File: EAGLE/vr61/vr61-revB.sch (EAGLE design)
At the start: 235 parts, among them J2 SM04B-SRSS-TB(LF)(SN), J6 MICROMOD-2222-C, Y1 74AHCT1G125

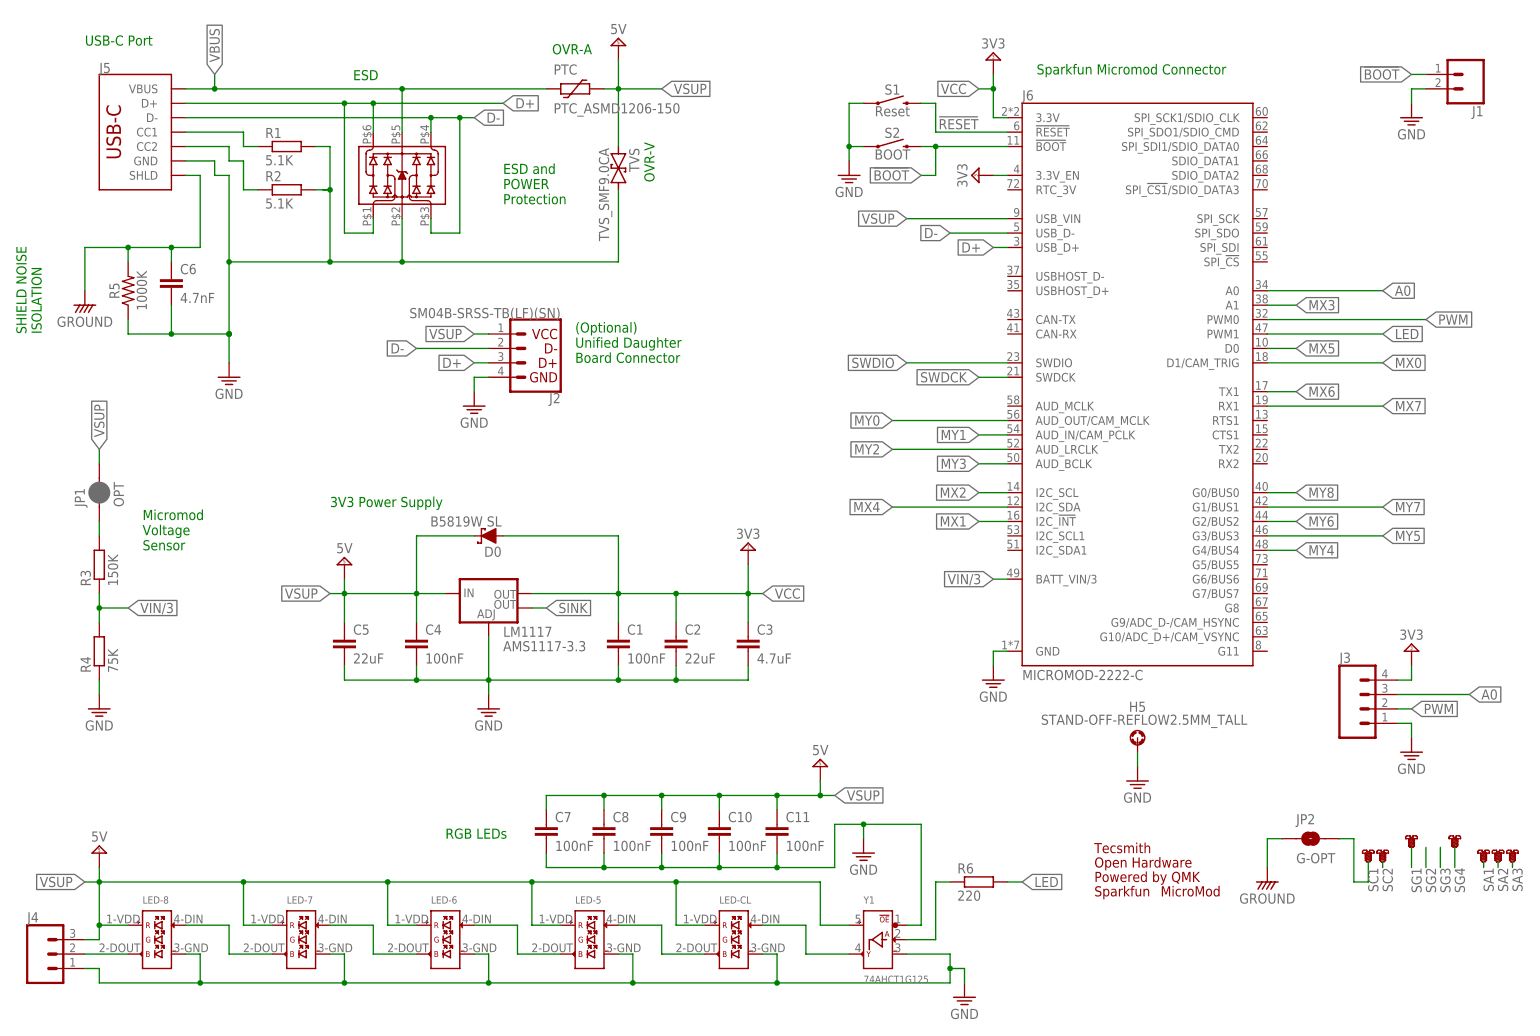
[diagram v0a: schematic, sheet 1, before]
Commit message: wip 2022-07-21
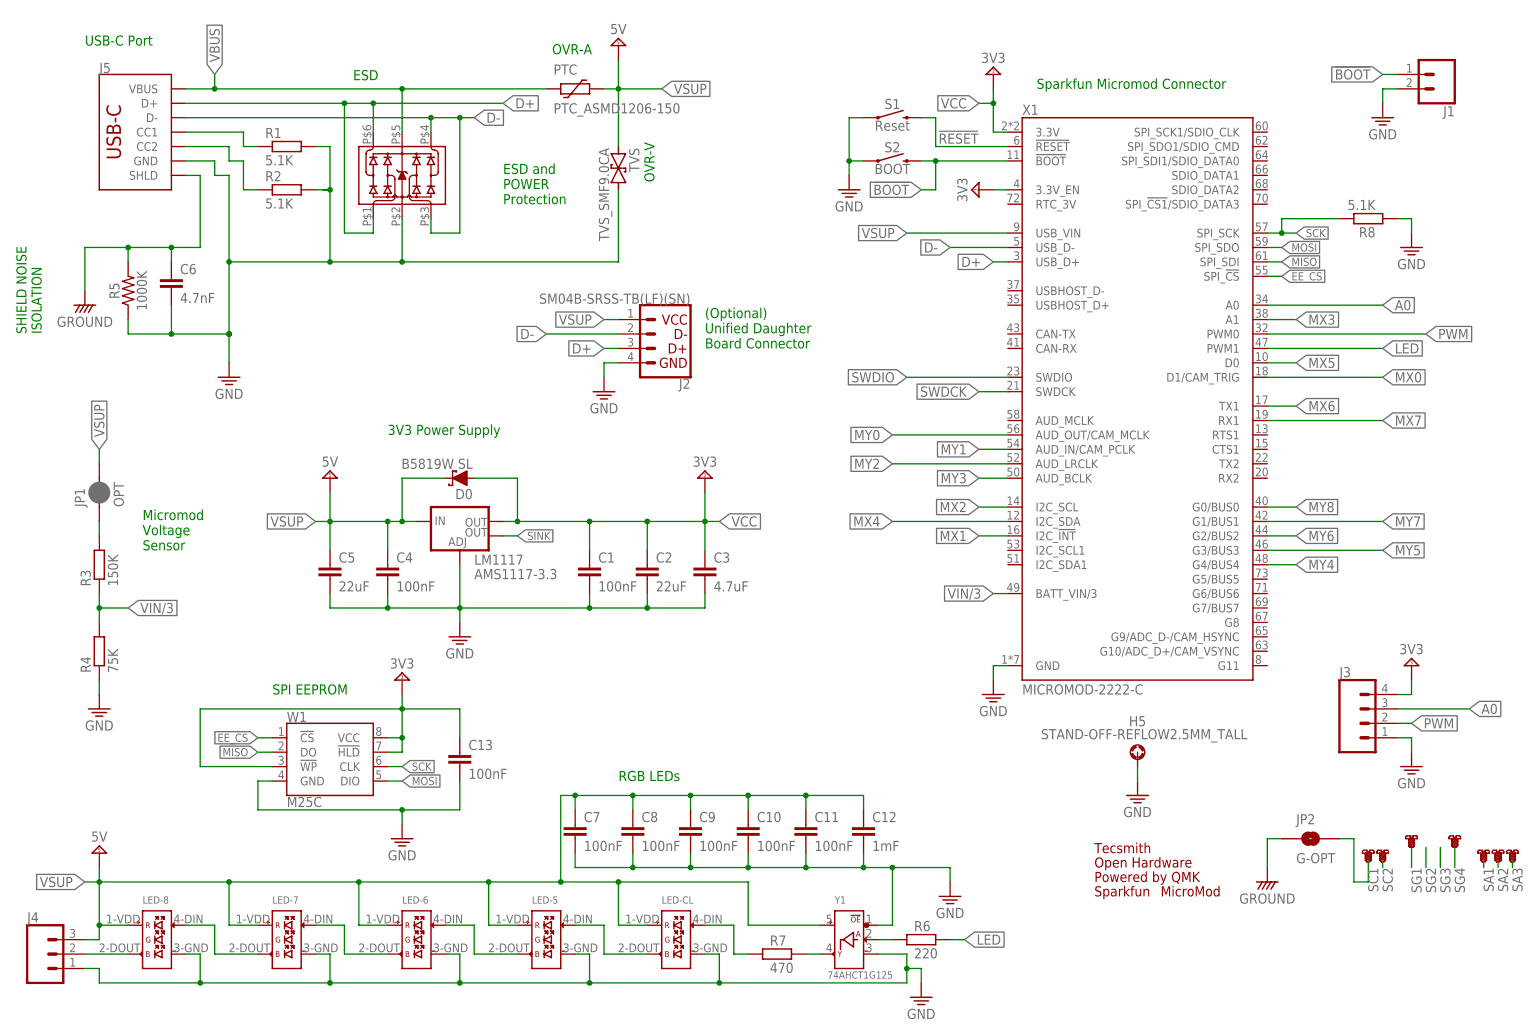
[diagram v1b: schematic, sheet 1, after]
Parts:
- removed J6: MICROMOD-2222-C, SparkFun-MicroMod:MICROMOD-2222-C
- added C12: 1mF, rcl:C-EUC0603
- added C13: 100nF, rcl:C-EUC0603
- added R7: 470, rcl:R-EU_R0603
- added R8: 5.1K, rcl:R-EU_R0603
- added W1: M25C, __untitled:M25C
- added X1: MICROMOD-2222-C, SparkFun-MicroMod:MICROMOD-2222-C
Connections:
- removed net N$70: LED-CL.4_DIN, Y1.Y_DOUT
- new net EE_CS: W1.!CS, X1.SPI_!CS!
- new net MISO: W1.DO, X1.SPI_SDI
- new net MOSI: W1.DIO, X1.SPI_SDO
- new net N$66: R7.2, Y1.Y_DOUT
- new net N$67: LED-CL.4_DIN, R7.1
- new net SCK: R8.2, W1.CLK, X1.SPI_SCK
- net !BOOT: now also X1.!BOOT!; no longer J6.!BOOT!
- net !RESET: now also X1.!RESET!; no longer J6.!RESET!
- net A0: now also X1.A0; no longer J6.A0
- net D+: now also X1.USB_D+; no longer J6.USB_D+
- net D-: now also X1.USB_D-; no longer J6.USB_D-
- net GND: now also C12.2, C13.2, R8.1, W1.GND, X1.GND; no longer J6.GND
- net LED: now also X1.PWM1; no longer J6.PWM1
- net MX0: now also X1.D1/CAM_TRIG; no longer J6.D1/CAM_TRIG
- net MX1: now also X1.I2C_!INT!; no longer J6.I2C_!INT!
- net MX2: now also X1.I2C_SCL; no longer J6.I2C_SCL
- net MX3: now also X1.A1; no longer J6.A1
- net MX4: now also X1.I2C_SDA; no longer J6.I2C_SDA
- net MX5: now also X1.D0; no longer J6.D0
- net MX6: now also X1.TX1; no longer J6.TX1
- net MX7: now also X1.RX1; no longer J6.RX1
- net MY0: now also X1.AUD_OUT/CAM_MCLK; no longer J6.AUD_OUT/CAM_MCLK
- net MY1: now also X1.AUD_IN/CAM_PCLK; no longer J6.AUD_IN/CAM_PCLK
- net MY2: now also X1.AUD_LRCLK; no longer J6.AUD_LRCLK
- net MY3: now also X1.AUD_BCLK; no longer J6.AUD_BCLK
- net MY4: now also X1.G4/BUS4; no longer J6.G4/BUS4
- net MY5: now also X1.G3/BUS3; no longer J6.G3/BUS3
- net MY6: now also X1.G2/BUS2; no longer J6.G2/BUS2
- net MY7: now also X1.G1/BUS1; no longer J6.G1/BUS1
- net MY8: now also X1.G0/BUS0; no longer J6.G0/BUS0
- net PWM: now also X1.PWM0; no longer J6.PWM0
- net SWDCK: now also X1.SWDCK; no longer J6.SWDCK
- net SWDIO: now also X1.SWDIO; no longer J6.SWDIO
- net VCC: now also C13.1, W1.!HLD, W1.!WP, W1.VCC, X1.3.3V, X1.3.3V_EN; no longer J6.3.3V, J6.3.3V_EN
- net VIN/3: now also X1.BATT_VIN/3; no longer J6.BATT_VIN/3
- net VSUP: now also C12.1, X1.USB_VIN; no longer J6.USB_VIN
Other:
- note added: "SPI EEPROM"
- moved on the sheet: C1, C10, C11, C2, C3, C4, C5, C7, C8, C9, D0, H5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
